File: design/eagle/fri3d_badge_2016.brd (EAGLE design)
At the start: 76.6 x 67.3 mm, 43 parts, among them Q1 MOSFET-NCHANNEL2N7002PW, U1 MCP73831

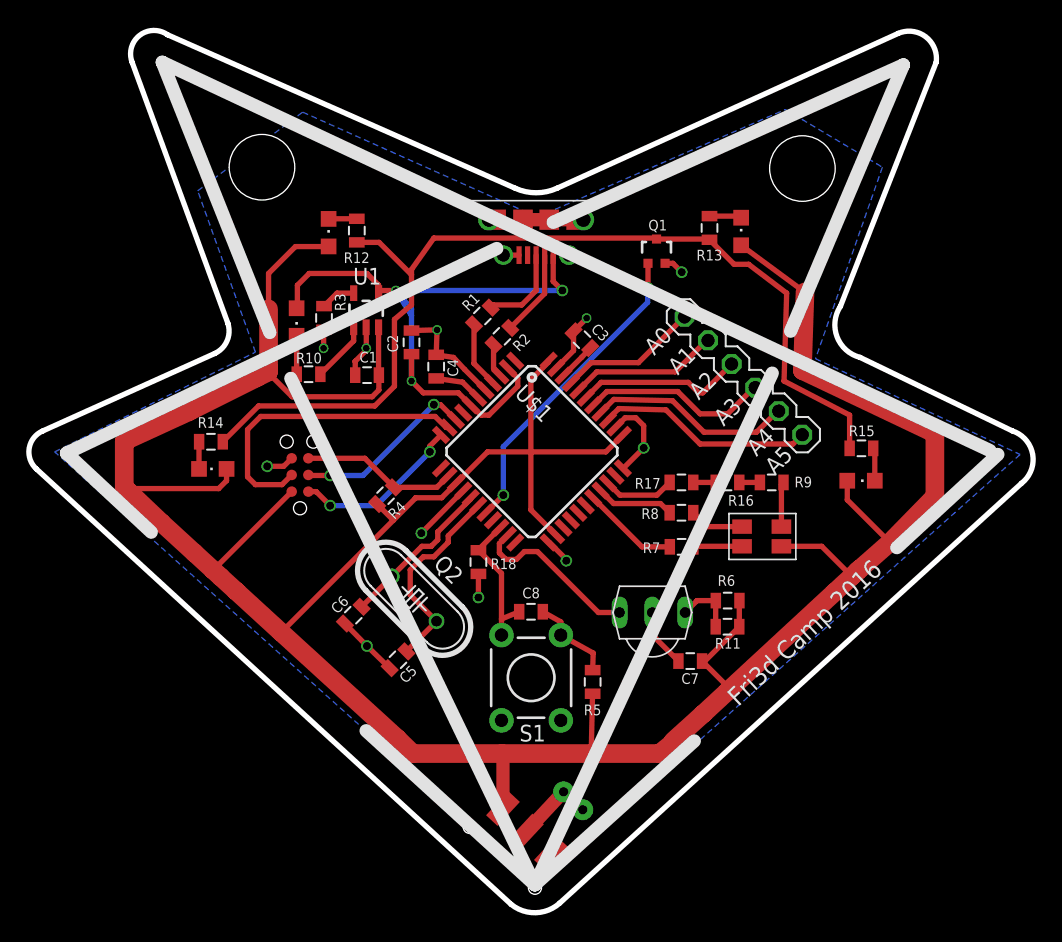
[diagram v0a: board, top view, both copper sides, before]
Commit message: added Fri3d Camp 2016 logo + silkscreen clean up
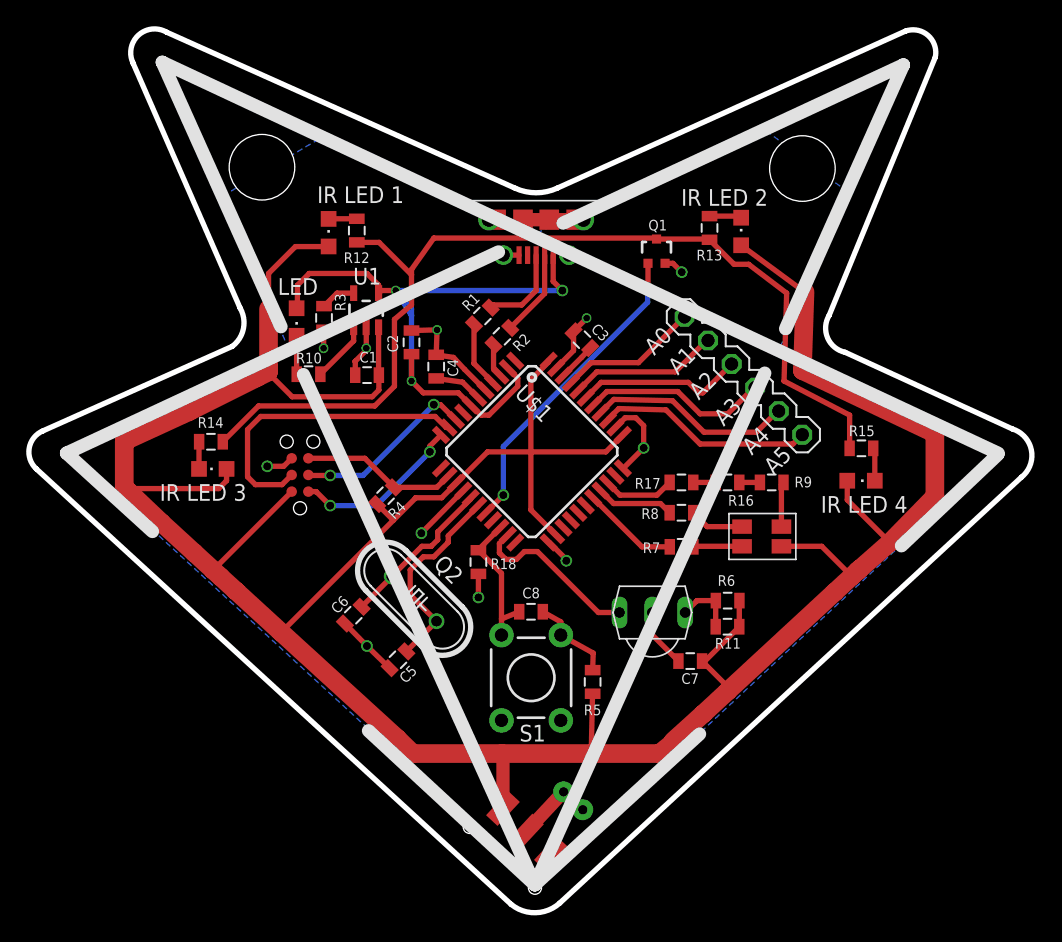
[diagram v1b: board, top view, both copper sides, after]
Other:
- board size 76.6 x 67.3 mm -> 76.5 x 67.4 mm
- board text removed: "Fri3d Camp 2016"
